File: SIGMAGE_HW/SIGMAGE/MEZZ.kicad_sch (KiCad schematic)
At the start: 2 parts, among them J12 61306421821, J8 61306421121

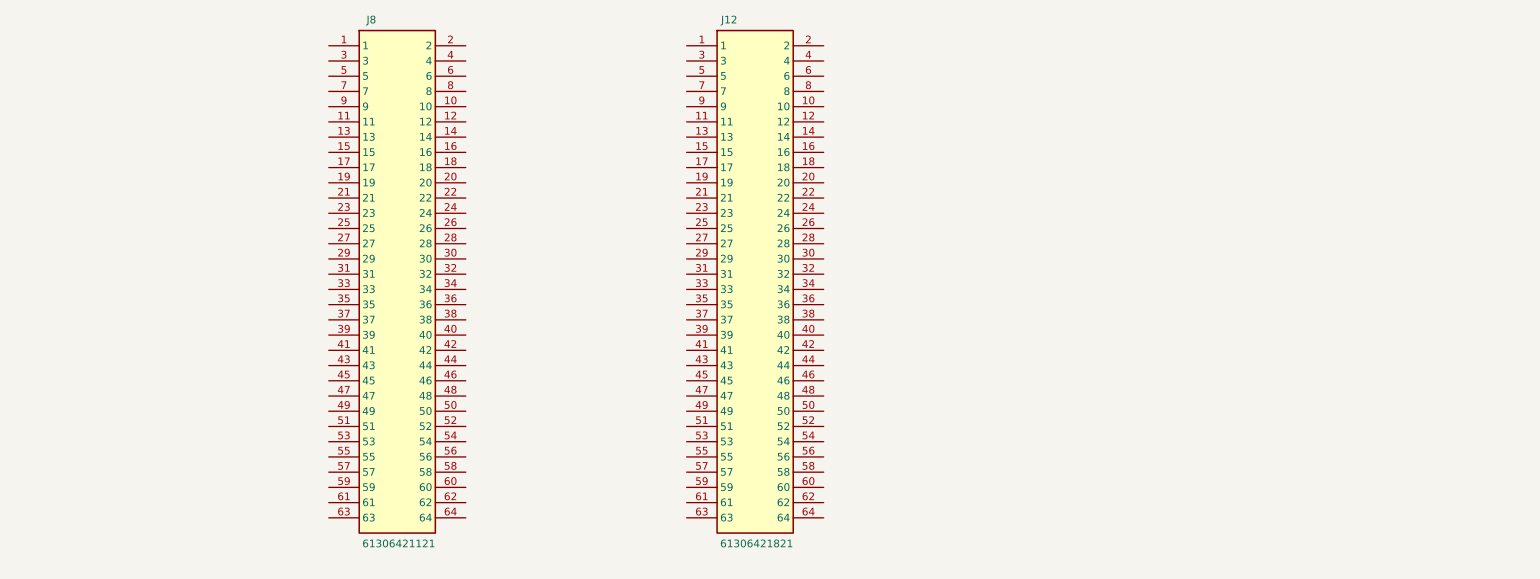
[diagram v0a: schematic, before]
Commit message: finished schematic
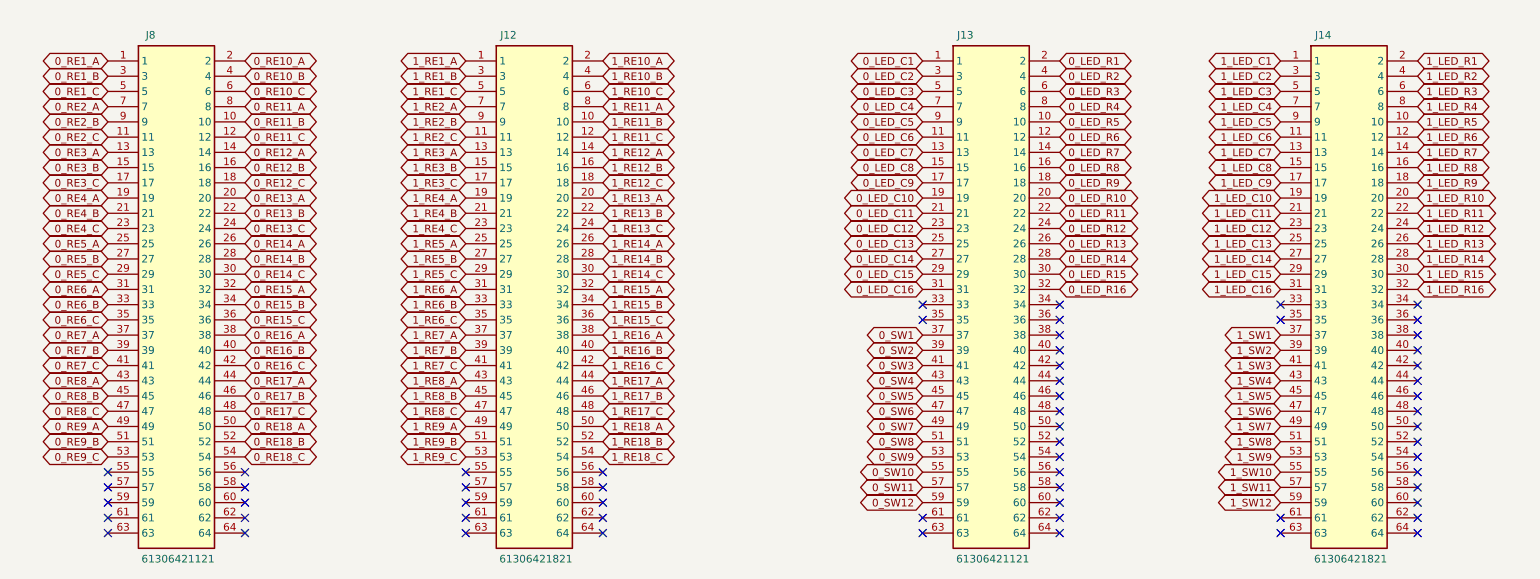
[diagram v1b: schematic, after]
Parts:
- added J13: 61306421121, SIGMAGE:61306421121, symbol SIGMAGE:61306421121
- added J14: 61306421821, SIGMAGE:61306421821, symbol SIGMAGE:61306421821
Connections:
- net 1_RE1_A: now reaches J12.1
- net 1_RE11_B: now reaches J12.10
- net 1_RE2_C: now reaches J12.11
- net 1_RE11_C: now reaches J12.12
- net 1_RE3_A: now reaches J12.13
- net 1_RE12_A: now reaches J12.14
- net 1_RE3_B: now reaches J12.15
- net 1_RE12_B: now reaches J12.16
- net 1_RE3_C: now reaches J12.17
- net 1_RE12_C: now reaches J12.18
- net 1_RE4_A: now reaches J12.19
- net 1_RE10_A: now reaches J12.2
- net 1_RE13_A: now reaches J12.20
- net 1_RE4_B: now reaches J12.21
- net 1_RE13_B: now reaches J12.22
- net 1_RE4_C: now reaches J12.23
- net 1_RE13_C: now reaches J12.24
- net 1_RE5_A: now reaches J12.25
- net 1_RE14_A: now reaches J12.26
- net 1_RE5_B: now reaches J12.27
- net 1_RE14_B: now reaches J12.28
- net 1_RE5_C: now reaches J12.29
- net 1_RE1_B: now reaches J12.3
- net 1_RE14_C: now reaches J12.30
- net 1_RE6_A: now reaches J12.31
- net 1_RE15_A: now reaches J12.32
- net 1_RE6_B: now reaches J12.33
- net 1_RE15_B: now reaches J12.34
- net 1_RE6_C: now reaches J12.35
- net 1_RE15_C: now reaches J12.36
- net 1_RE7_A: now reaches J12.37
- net 1_RE16_A: now reaches J12.38
- net 1_RE7_B: now reaches J12.39
- net 1_RE10_B: now reaches J12.4
- net 1_RE16_B: now reaches J12.40
- net 1_RE7_C: now reaches J12.41
- net 1_RE16_C: now reaches J12.42
- net 1_RE8_A: now reaches J12.43
- net 1_RE17_A: now reaches J12.44
- net 1_RE8_B: now reaches J12.45
- net 1_RE17_B: now reaches J12.46
- net 1_RE8_C: now reaches J12.47
- net 1_RE17_C: now reaches J12.48
- net 1_RE9_A: now reaches J12.49
- net 1_RE1_C: now reaches J12.5
- net 1_RE18_A: now reaches J12.50
- net 1_RE9_B: now reaches J12.51
- net 1_RE18_B: now reaches J12.52
- net 1_RE9_C: now reaches J12.53
- net 1_RE18_C: now reaches J12.54
- net 1_RE10_C: now reaches J12.6
- net 1_RE2_A: now reaches J12.7
- net 1_RE11_A: now reaches J12.8
- net 1_RE2_B: now reaches J12.9
- net 0_RE1_A: now reaches J8.1
- net 0_RE11_B: now reaches J8.10
- net 0_RE2_C: now reaches J8.11
- net 0_RE11_C: now reaches J8.12
- net 0_RE3_A: now reaches J8.13
- net 0_RE12_A: now reaches J8.14
- net 0_RE3_B: now reaches J8.15
- net 0_RE12_B: now reaches J8.16
- net 0_RE3_C: now reaches J8.17
- net 0_RE12_C: now reaches J8.18
- net 0_RE4_A: now reaches J8.19
- net 0_RE10_A: now reaches J8.2
- net 0_RE13_A: now reaches J8.20
- net 0_RE4_B: now reaches J8.21
- net 0_RE13_B: now reaches J8.22
- net 0_RE4_C: now reaches J8.23
- net 0_RE13_C: now reaches J8.24
- net 0_RE5_A: now reaches J8.25
- net 0_RE14_A: now reaches J8.26
- net 0_RE5_B: now reaches J8.27
- net 0_RE14_B: now reaches J8.28
- net 0_RE5_C: now reaches J8.29
- net 0_RE1_B: now reaches J8.3
- net 0_RE14_C: now reaches J8.30
- net 0_RE6_A: now reaches J8.31
- net 0_RE15_A: now reaches J8.32
- net 0_RE6_B: now reaches J8.33
- net 0_RE15_B: now reaches J8.34
- net 0_RE6_C: now reaches J8.35
- net 0_RE15_C: now reaches J8.36
- net 0_RE7_A: now reaches J8.37
- net 0_RE16_A: now reaches J8.38
- net 0_RE7_B: now reaches J8.39
- net 0_RE10_B: now reaches J8.4
- net 0_RE16_B: now reaches J8.40
- net 0_RE7_C: now reaches J8.41
- net 0_RE16_C: now reaches J8.42
- net 0_RE8_A: now reaches J8.43
- net 0_RE17_A: now reaches J8.44
- net 0_RE8_B: now reaches J8.45
- net 0_RE17_B: now reaches J8.46
- net 0_RE8_C: now reaches J8.47
- net 0_RE17_C: now reaches J8.48
- net 0_RE9_A: now reaches J8.49
- net 0_RE1_C: now reaches J8.5
- net 0_RE18_A: now reaches J8.50
- net 0_RE9_B: now reaches J8.51
- net 0_RE18_B: now reaches J8.52
- net 0_RE9_C: now reaches J8.53
- net 0_RE18_C: now reaches J8.54
- net 0_RE10_C: now reaches J8.6
- net 0_RE2_A: now reaches J8.7
- net 0_RE11_A: now reaches J8.8
- net 0_RE2_B: now reaches J8.9
- new net 0_LED_C1: J13.1
- new net 0_LED_C10: J13.19
- new net 0_LED_C11: J13.21
- new net 0_LED_C12: J13.23
- new net 0_LED_C13: J13.25
- new net 0_LED_C14: J13.27
- new net 0_LED_C15: J13.29
- new net 0_LED_C16: J13.31
- new net 0_LED_C2: J13.3
- new net 0_LED_C3: J13.5
- new net 0_LED_C4: J13.7
- new net 0_LED_C5: J13.9
- new net 0_LED_C6: J13.11
- new net 0_LED_C7: J13.13
- new net 0_LED_C8: J13.15
- new net 0_LED_C9: J13.17
- new net 0_LED_R1: J13.2
- new net 0_LED_R10: J13.20
- new net 0_LED_R11: J13.22
- new net 0_LED_R12: J13.24
- new net 0_LED_R13: J13.26
- new net 0_LED_R14: J13.28
- new net 0_LED_R15: J13.30
- new net 0_LED_R16: J13.32
- new net 0_LED_R2: J13.4
- new net 0_LED_R3: J13.6
- new net 0_LED_R4: J13.8
- new net 0_LED_R5: J13.10
- new net 0_LED_R6: J13.12
- new net 0_LED_R7: J13.14
- new net 0_LED_R8: J13.16
- new net 0_LED_R9: J13.18
- new net 0_SW1: J13.37
- new net 0_SW10: J13.55
- new net 0_SW11: J13.57
- new net 0_SW12: J13.59
- new net 0_SW2: J13.39
- new net 0_SW3: J13.41
- new net 0_SW4: J13.43
- new net 0_SW5: J13.45
- new net 0_SW6: J13.47
- new net 0_SW7: J13.49
- new net 0_SW8: J13.51
- new net 0_SW9: J13.53
- new net 1_LED_C1: J14.1
- new net 1_LED_C10: J14.19
- new net 1_LED_C11: J14.21
- new net 1_LED_C12: J14.23
- new net 1_LED_C13: J14.25
- new net 1_LED_C14: J14.27
- new net 1_LED_C15: J14.29
- new net 1_LED_C16: J14.31
- new net 1_LED_C2: J14.3
- new net 1_LED_C3: J14.5
- new net 1_LED_C4: J14.7
- new net 1_LED_C5: J14.9
- new net 1_LED_C6: J14.11
- new net 1_LED_C7: J14.13
- new net 1_LED_C8: J14.15
- new net 1_LED_C9: J14.17
- new net 1_LED_R1: J14.2
- new net 1_LED_R10: J14.20
- new net 1_LED_R11: J14.22
- new net 1_LED_R12: J14.24
- new net 1_LED_R13: J14.26
- new net 1_LED_R14: J14.28
- new net 1_LED_R15: J14.30
- new net 1_LED_R16: J14.32
- new net 1_LED_R2: J14.4
- new net 1_LED_R3: J14.6
- new net 1_LED_R4: J14.8
- new net 1_LED_R5: J14.10
- new net 1_LED_R6: J14.12
- new net 1_LED_R7: J14.14
- new net 1_LED_R8: J14.16
- new net 1_LED_R9: J14.18
- new net 1_SW1: J14.37
- new net 1_SW10: J14.55
- new net 1_SW11: J14.57
- new net 1_SW12: J14.59
- new net 1_SW2: J14.39
- new net 1_SW3: J14.41
- new net 1_SW4: J14.43
- new net 1_SW5: J14.45
- new net 1_SW6: J14.47
- new net 1_SW7: J14.49
- new net 1_SW8: J14.51
- new net 1_SW9: J14.53
- no-connect marks 0 -> 60
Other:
- moved on the sheet: J12, J8

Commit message: basic layout
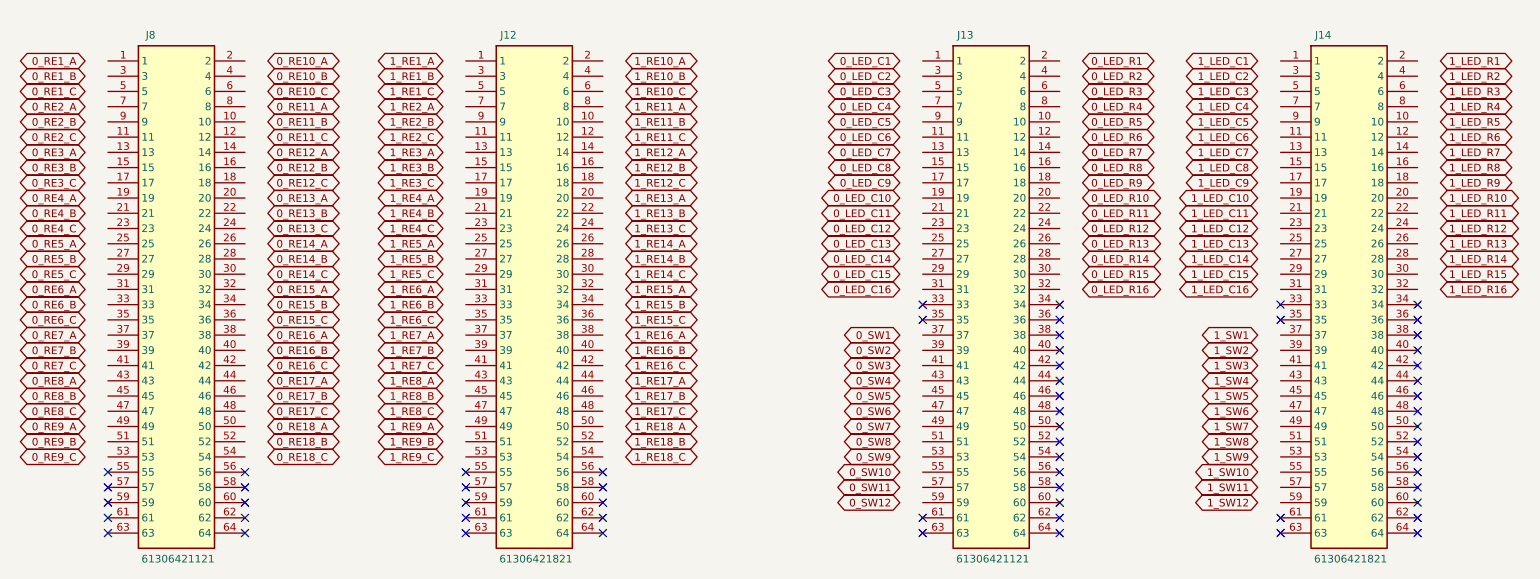
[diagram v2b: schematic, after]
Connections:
- net 0_LED_C1: no longer J13.1
- net 0_LED_C10: no longer J13.19
- net 0_LED_C11: no longer J13.21
- net 0_LED_C12: no longer J13.23
- net 0_LED_C13: no longer J13.25
- net 0_LED_C14: no longer J13.27
- net 0_LED_C15: no longer J13.29
- net 0_LED_C16: no longer J13.31
- net 0_LED_C2: no longer J13.3
- net 0_LED_C3: no longer J13.5
- net 0_LED_C4: no longer J13.7
- net 0_LED_C5: no longer J13.9
- net 0_LED_C6: no longer J13.11
- net 0_LED_C7: no longer J13.13
- net 0_LED_C8: no longer J13.15
- net 0_LED_C9: no longer J13.17
- net 0_LED_R1: no longer J13.2
- net 0_LED_R10: no longer J13.20
- net 0_LED_R11: no longer J13.22
- net 0_LED_R12: no longer J13.24
- net 0_LED_R13: no longer J13.26
- net 0_LED_R14: no longer J13.28
- net 0_LED_R15: no longer J13.30
- net 0_LED_R16: no longer J13.32
- net 0_LED_R2: no longer J13.4
- net 0_LED_R3: no longer J13.6
- net 0_LED_R4: no longer J13.8
- net 0_LED_R5: no longer J13.10
- net 0_LED_R6: no longer J13.12
- net 0_LED_R7: no longer J13.14
- net 0_LED_R8: no longer J13.16
- net 0_LED_R9: no longer J13.18
- net 0_RE10_A: no longer J8.2
- net 0_RE10_B: no longer J8.4
- net 0_RE10_C: no longer J8.6
- net 0_RE11_A: no longer J8.8
- net 0_RE11_B: no longer J8.10
- net 0_RE11_C: no longer J8.12
- net 0_RE12_A: no longer J8.14
- net 0_RE12_B: no longer J8.16
- net 0_RE12_C: no longer J8.18
- net 0_RE13_A: no longer J8.20
- net 0_RE13_B: no longer J8.22
- net 0_RE13_C: no longer J8.24
- net 0_RE14_A: no longer J8.26
- net 0_RE14_B: no longer J8.28
- net 0_RE14_C: no longer J8.30
- net 0_RE15_A: no longer J8.32
- net 0_RE15_B: no longer J8.34
- net 0_RE15_C: no longer J8.36
- net 0_RE16_A: no longer J8.38
- net 0_RE16_B: no longer J8.40
- net 0_RE16_C: no longer J8.42
- net 0_RE17_A: no longer J8.44
- net 0_RE17_B: no longer J8.46
- net 0_RE17_C: no longer J8.48
- net 0_RE18_A: no longer J8.50
- net 0_RE18_B: no longer J8.52
- net 0_RE18_C: no longer J8.54
- net 0_RE1_A: no longer J8.1
- net 0_RE1_B: no longer J8.3
- net 0_RE1_C: no longer J8.5
- net 0_RE2_A: no longer J8.7
- net 0_RE2_B: no longer J8.9
- net 0_RE2_C: no longer J8.11
- net 0_RE3_A: no longer J8.13
- net 0_RE3_B: no longer J8.15
- net 0_RE3_C: no longer J8.17
- net 0_RE4_A: no longer J8.19
- net 0_RE4_B: no longer J8.21
- net 0_RE4_C: no longer J8.23
- net 0_RE5_A: no longer J8.25
- net 0_RE5_B: no longer J8.27
- net 0_RE5_C: no longer J8.29
- net 0_RE6_A: no longer J8.31
- net 0_RE6_B: no longer J8.33
- net 0_RE6_C: no longer J8.35
- net 0_RE7_A: no longer J8.37
- net 0_RE7_B: no longer J8.39
- net 0_RE7_C: no longer J8.41
- net 0_RE8_A: no longer J8.43
- net 0_RE8_B: no longer J8.45
- net 0_RE8_C: no longer J8.47
- net 0_RE9_A: no longer J8.49
- net 0_RE9_B: no longer J8.51
- net 0_RE9_C: no longer J8.53
- net 0_SW1: no longer J13.37
- net 0_SW10: no longer J13.55
- net 0_SW11: no longer J13.57
- net 0_SW12: no longer J13.59
- net 0_SW2: no longer J13.39
- net 0_SW3: no longer J13.41
- net 0_SW4: no longer J13.43
- net 0_SW5: no longer J13.45
- net 0_SW6: no longer J13.47
- net 0_SW7: no longer J13.49
- net 0_SW8: no longer J13.51
- net 0_SW9: no longer J13.53
- net 1_LED_C1: no longer J14.1
- net 1_LED_C10: no longer J14.19
- net 1_LED_C11: no longer J14.21
- net 1_LED_C12: no longer J14.23
- net 1_LED_C13: no longer J14.25
- net 1_LED_C14: no longer J14.27
- net 1_LED_C15: no longer J14.29
- net 1_LED_C16: no longer J14.31
- net 1_LED_C2: no longer J14.3
- net 1_LED_C3: no longer J14.5
- net 1_LED_C4: no longer J14.7
- net 1_LED_C5: no longer J14.9
- net 1_LED_C6: no longer J14.11
- net 1_LED_C7: no longer J14.13
- net 1_LED_C8: no longer J14.15
- net 1_LED_C9: no longer J14.17
- net 1_LED_R1: no longer J14.2
- net 1_LED_R10: no longer J14.20
- net 1_LED_R11: no longer J14.22
- net 1_LED_R12: no longer J14.24
- net 1_LED_R13: no longer J14.26
- net 1_LED_R14: no longer J14.28
- net 1_LED_R15: no longer J14.30
- net 1_LED_R16: no longer J14.32
- net 1_LED_R2: no longer J14.4
- net 1_LED_R3: no longer J14.6
- net 1_LED_R4: no longer J14.8
- net 1_LED_R5: no longer J14.10
- net 1_LED_R6: no longer J14.12
- net 1_LED_R7: no longer J14.14
- net 1_LED_R8: no longer J14.16
- net 1_LED_R9: no longer J14.18
- net 1_RE10_A: no longer J12.2
- net 1_RE10_B: no longer J12.4
- net 1_RE10_C: no longer J12.6
- net 1_RE11_A: no longer J12.8
- net 1_RE11_B: no longer J12.10
- net 1_RE11_C: no longer J12.12
- net 1_RE12_A: no longer J12.14
- net 1_RE12_B: no longer J12.16
- net 1_RE12_C: no longer J12.18
- net 1_RE13_A: no longer J12.20
- net 1_RE13_B: no longer J12.22
- net 1_RE13_C: no longer J12.24
- net 1_RE14_A: no longer J12.26
- net 1_RE14_B: no longer J12.28
- net 1_RE14_C: no longer J12.30
- net 1_RE15_A: no longer J12.32
- net 1_RE15_B: no longer J12.34
- net 1_RE15_C: no longer J12.36
- net 1_RE16_A: no longer J12.38
- net 1_RE16_B: no longer J12.40
- net 1_RE16_C: no longer J12.42
- net 1_RE17_A: no longer J12.44
- net 1_RE17_B: no longer J12.46
- net 1_RE17_C: no longer J12.48
- net 1_RE18_A: no longer J12.50
- net 1_RE18_B: no longer J12.52
- net 1_RE18_C: no longer J12.54
- net 1_RE1_A: no longer J12.1
- net 1_RE1_B: no longer J12.3
- net 1_RE1_C: no longer J12.5
- net 1_RE2_A: no longer J12.7
- net 1_RE2_B: no longer J12.9
- net 1_RE2_C: no longer J12.11
- net 1_RE3_A: no longer J12.13
- net 1_RE3_B: no longer J12.15
- net 1_RE3_C: no longer J12.17
- net 1_RE4_A: no longer J12.19
- net 1_RE4_B: no longer J12.21
- net 1_RE4_C: no longer J12.23
- net 1_RE5_A: no longer J12.25
- net 1_RE5_B: no longer J12.27
- net 1_RE5_C: no longer J12.29
- net 1_RE6_A: no longer J12.31
- net 1_RE6_B: no longer J12.33
- net 1_RE6_C: no longer J12.35
- net 1_RE7_A: no longer J12.37
- net 1_RE7_B: no longer J12.39
- net 1_RE7_C: no longer J12.41
- net 1_RE8_A: no longer J12.43
- net 1_RE8_B: no longer J12.45
- net 1_RE8_C: no longer J12.47
- net 1_RE9_A: no longer J12.49
- net 1_RE9_B: no longer J12.51
- net 1_RE9_C: no longer J12.53
- net 1_SW1: no longer J14.37
- net 1_SW10: no longer J14.55
- net 1_SW11: no longer J14.57
- net 1_SW12: no longer J14.59
- net 1_SW2: no longer J14.39
- net 1_SW3: no longer J14.41
- net 1_SW4: no longer J14.43
- net 1_SW5: no longer J14.45
- net 1_SW6: no longer J14.47
- net 1_SW7: no longer J14.49
- net 1_SW8: no longer J14.51
- net 1_SW9: no longer J14.53
